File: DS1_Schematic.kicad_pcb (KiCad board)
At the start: 2 copper layers, 81.8 x 63.5 mm, 58 parts, among them J1 AudioJack3_Switch, J2 AudioJack2_Switch, J3 BAT_CON, J4 PWR_SUPP_COM, Q1 2SC2240, Q2 2SC2240, Q3 2SC2240, U1 NE5532

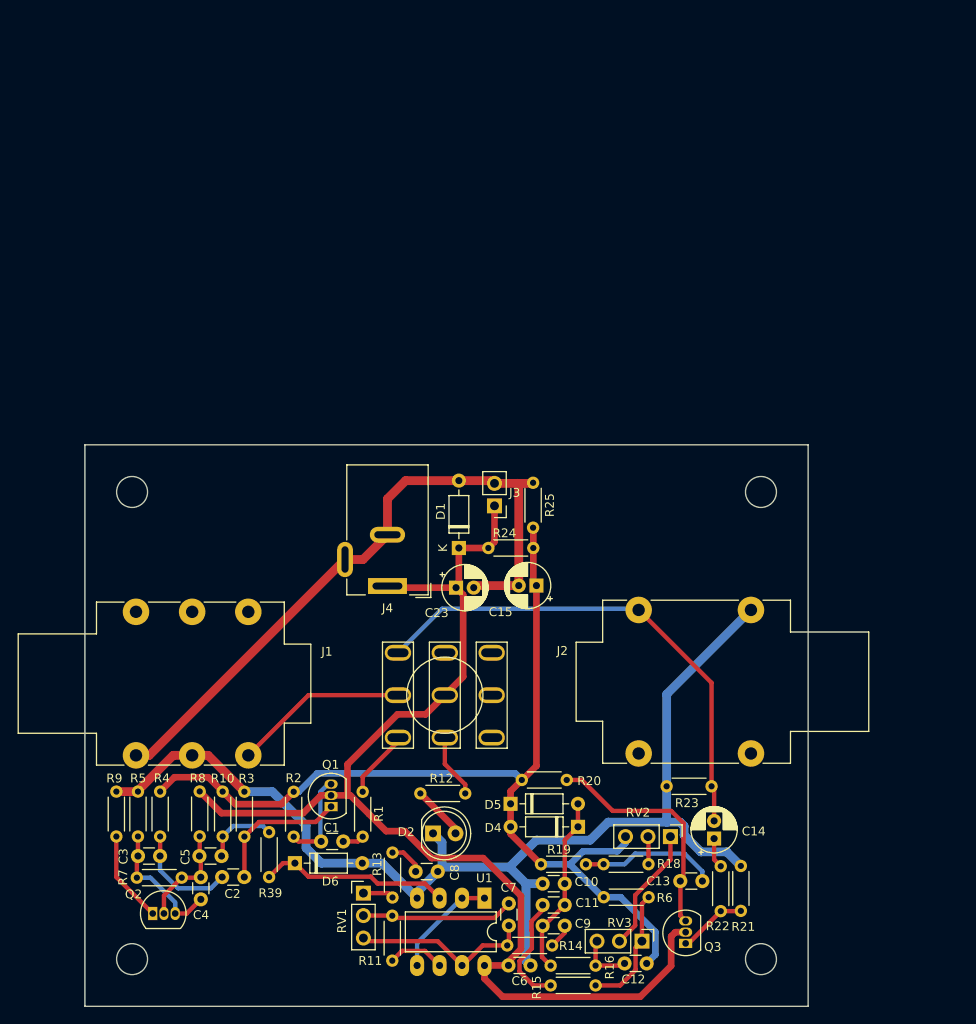
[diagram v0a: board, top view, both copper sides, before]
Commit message: updated THT
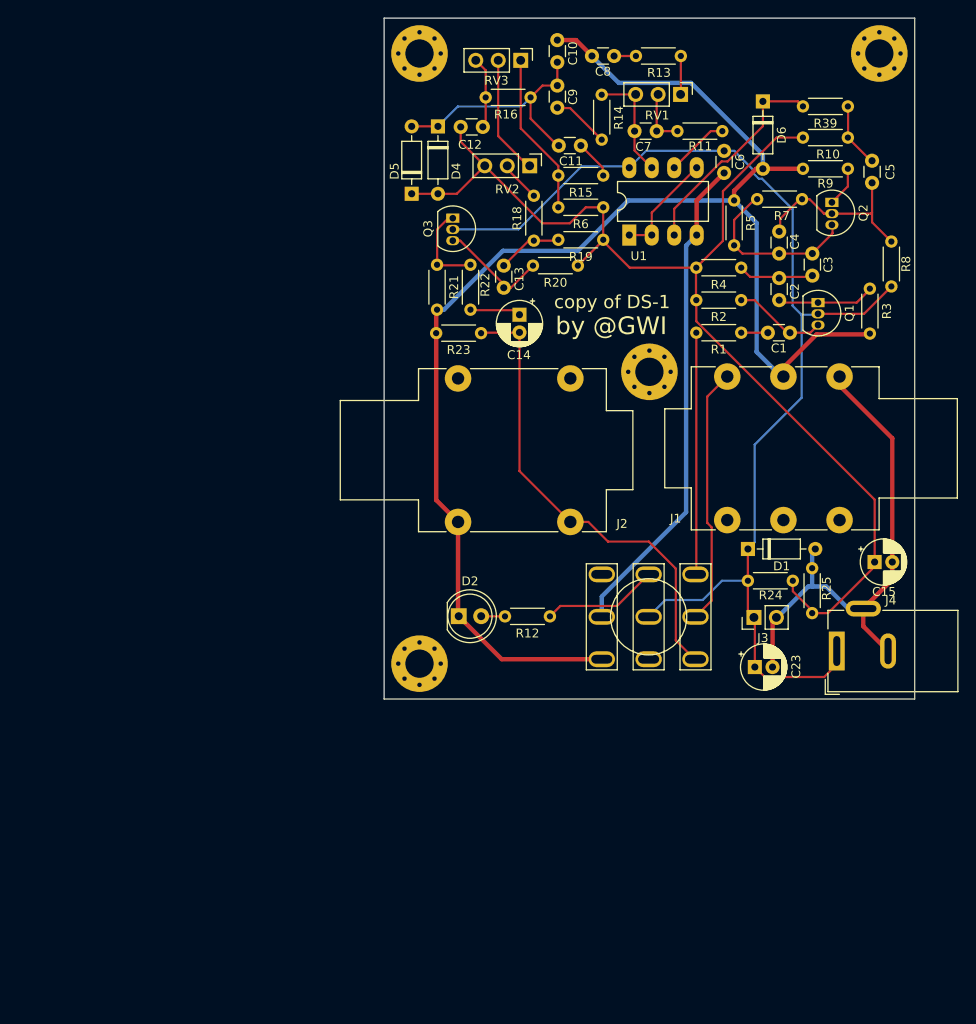
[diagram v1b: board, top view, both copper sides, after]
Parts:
- added REF**: MountingHole_3.2mm_M3_Pad_Via, MountingHole:MountingHole_3.2mm_M3_Pad_Via, F.Cu at (90.0, 103.0)
- added REF**: MountingHole_3.2mm_M3_Pad_Via, MountingHole:MountingHole_3.2mm_M3_Pad_Via, F.Cu at (64.0, 67.0)
- added REF**: MountingHole_3.2mm_M3_Pad_Via, MountingHole:MountingHole_3.2mm_M3_Pad_Via, F.Cu at (116.0, 67.0)
- added REF**: MountingHole_3.2mm_M3_Pad_Via, MountingHole:MountingHole_3.2mm_M3_Pad_Via, F.Cu at (64.0, 136.0)
- moved R9 112.0 mm to (112.4, 80.0), turned to 180 degrees
- moved Q2 111.2 mm to (110.6, 83.8), turned to -90 degrees
- moved C5 107.7 mm to (115.2, 79.1), turned to -90 degrees
- moved R39 105.0 mm to (112.4, 73.0), turned to 180 degrees
- moved R7 104.0 mm to (102.2, 83.5)
- moved R8 103.2 mm to (117.4, 88.3), turned to -90 degrees
- moved C3 102.3 mm to (108.4, 89.6), turned to -90 degrees
- moved D6 101.1 mm to (102.8, 72.4), turned to -90 degrees
- moved R11 101.0 mm to (98.2, 75.8), turned to 180 degrees
- moved RV3 100.6 mm to (75.4, 67.8)
- moved R10 98.9 mm to (107.4, 76.5), turned to 0 degrees
- moved R16 98.2 mm to (76.6, 72.0), turned to 180 degrees
- moved C4 98.0 mm to (104.7, 89.6)
- moved RV1 97.2 mm to (93.5, 71.6), turned to -90 degrees
- moved C12 96.9 mm to (68.7, 75.3), turned to 0 degrees
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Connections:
- C6 pad 2: GND -> Net-(C6-Pad2)
- S1 pad P$7: unconnected-(S1-PadP$7) -> GND
- S1 pad P$8: unconnected-(S1-PadP$8) -> Net-(C6-Pad2)
- U1 pad 4: GND -> Net-(C6-Pad2)
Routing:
- net Net-(C6-Pad2): track 0.00 -> 55.9 mm
- net GND: track 133.2 -> 167.5 mm
- net Net-(R1-Pad1): track 7.91 -> 27.3 mm
- net GND1: track 77.1 -> 58.6 mm
- net +4.5V: track 113.6 -> 129.4 mm
- net Net-(C13-Pad1): track 26.7 -> 12.5 mm
- net Net-(C7-Pad2): track 17.1 -> 6.56 mm
- net Net-(C4-Pad2): track 11.7 -> 21.0 mm
- net Net-(J1-PadT): track 19.7 -> 29.1 mm
- net Net-(C11-Pad2): track 12.8 -> 4.42 mm
- net Net-(C13-Pad2): track 15.6 -> 7.38 mm
- net Op-Amp Output: track 20.6 -> 27.9 mm
- net Net-(C7-Pad1): track 20.0 -> 13.0 mm
- net Net-(Q2-Pad1): track 10.4 -> 4.55 mm
- net Net-(R12-Pad1): track 7.27 -> 13.1 mm
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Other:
- board size 81.8 x 63.5 mm -> 60 x 77 mm
- board text added: "by @GWI"
- board text added: "copy of DS-1"
